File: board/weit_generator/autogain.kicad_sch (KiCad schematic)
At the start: 10 parts, among them U1 MCP6004, U3 LM4041LP-ADJ

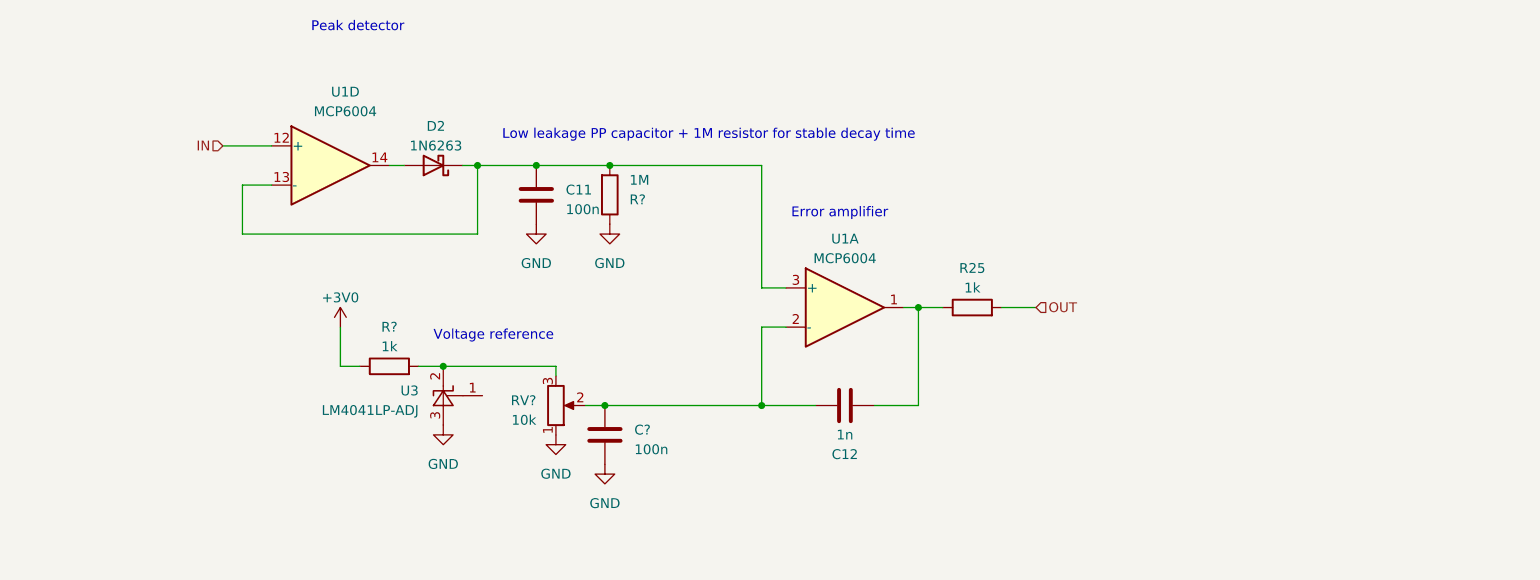
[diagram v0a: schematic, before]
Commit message: hopefully repaired instability
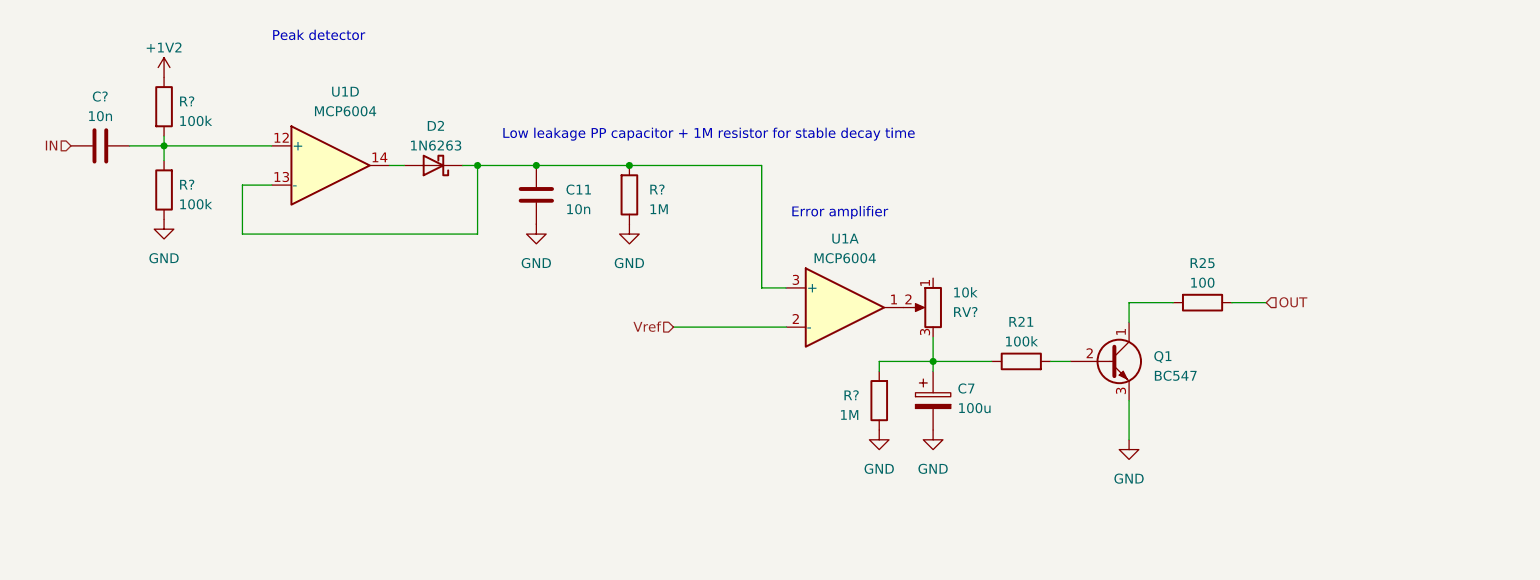
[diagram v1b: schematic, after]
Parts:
- removed C12: 1n, Capacitor_SMD:C_0805_2012Metric_Pad1.18x1.45mm_HandSolder, symbol Device:C
- removed C?: 100n, Capacitor_SMD:C_0805_2012Metric_Pad1.18x1.45mm_HandSolder, symbol Device:C
- removed R?: 1k, Resistor_SMD:R_0805_2012Metric_Pad1.20x1.40mm_HandSolder, symbol Device:R
- removed RV?: 10k, Potentiometer_THT:Potentiometer_Bourns_3266Y_Vertical, symbol Device:R_Potentiometer
- removed U3: LM4041LP-ADJ, Package_TO_SOT_THT:TO-92_Inline, symbol Reference_Voltage:LM4041LP-ADJ
- added C7: 100u, symbol Device:C_Polarized
- added C?: 10n, Capacitor_THT:C_Rect_L9.0mm_W4.0mm_P7.50mm_MKT, symbol Device:C
- added Q1: BC547, Package_TO_SOT_THT:TO-92_Inline, symbol Transistor_BJT:BC547
- added R21: 100k, Resistor_THT:R_Axial_DIN0207_L6.3mm_D2.5mm_P2.54mm_Vertical, symbol Device:R
- added R?: 1M, Resistor_THT:R_Axial_DIN0207_L6.3mm_D2.5mm_P2.54mm_Vertical, symbol Device:R
- added R? (x2): 100k, Resistor_SMD:R_0805_2012Metric_Pad1.20x1.40mm_HandSolder, symbol Device:R
- added RV?: 10k, Potentiometer_THT:Potentiometer_Bourns_3266Y_Vertical, symbol Device:R_Potentiometer
- C11: value 100n -> 10n
- R25: value 1k -> 100
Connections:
- net GND: now also C7.2, Q1.3 (E), R?.1, R?.1
- net IN: now also C?.2; no longer U1.12 (+)
- net OUT: now also R25.1; no longer R25.2
- net at U1.1: now also RV?.2; no longer R25.1
- net Vref: now reaches U1.2 (-)
- new net: C7.1, R21.1, R?.2, RV?.3
- new net: C?.1, R?.2, R?.2, U1.12 (+)
- new net: Q1.1 (C), R25.2
- new net: Q1.2 (B), R21.2
- new net +1V2: R?.1
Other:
- note removed: "Voltage reference"
- moved on the sheet: R25, R?

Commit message: New layout
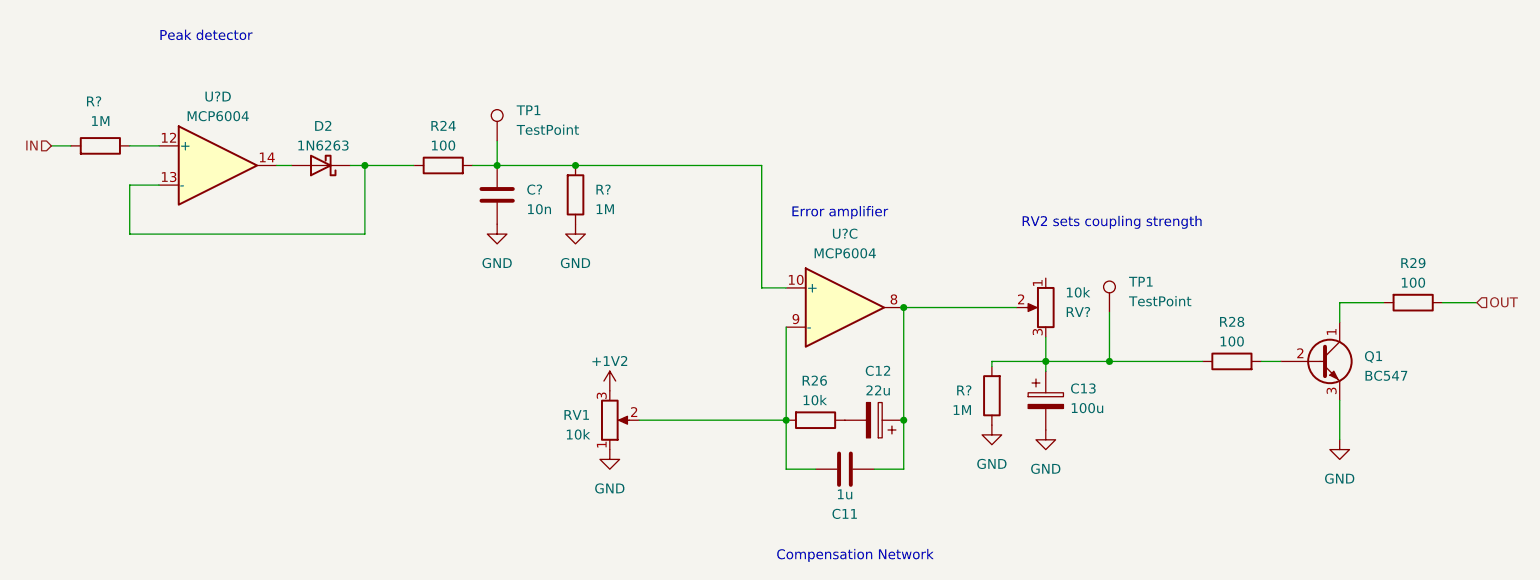
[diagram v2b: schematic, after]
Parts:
- removed C?: 10n, Capacitor_THT:C_Rect_L9.0mm_W4.0mm_P7.50mm_MKT, symbol Device:C
- removed R? (x2): 100k, Resistor_SMD:R_0805_2012Metric_Pad1.20x1.40mm_HandSolder, symbol Device:R
- removed U1: MCP6004, Package_DIP:DIP-14_W7.62mm_Socket_LongPads, symbol Amplifier_Operational:MCP6004
- added C11: 1u, Capacitor_THT:C_Rect_L7.2mm_W4.5mm_P5.00mm_FKS2_FKP2_MKS2_MKP2, symbol Device:C
- added C12: 22u, Capacitor_THT:CP_Radial_D6.3mm_P2.50mm, symbol Device:C_Polarized
- added R24: 100, Resistor_THT:R_Axial_DIN0207_L6.3mm_D2.5mm_P2.54mm_Vertical, symbol Device:R
- added R26: 10k, Resistor_THT:R_Axial_DIN0207_L6.3mm_D2.5mm_P2.54mm_Vertical, symbol Device:R
- added R?: 1M, Resistor_THT:R_Axial_DIN0207_L6.3mm_D2.5mm_P2.54mm_Vertical, symbol Device:R
- added RV1: 10k, Potentiometer_THT:Potentiometer_Bourns_3266Y_Vertical, symbol Device:R_Potentiometer
- added TP1 (x2): TestPoint, TestPoint:TestPoint_Pad_D3.0mm, symbol Connector:TestPoint
- added U? (x2): MCP6004, Package_DIP:DIP-14_W7.62mm_Socket, symbol Amplifier_Operational:MCP6004
- C13: renamed from C7; footprint (none) -> Capacitor_THT:CP_Radial_D6.3mm_P2.50mm
- C?: renamed from C11; footprint Capacitor_THT:C_Rect_L13.0mm_W6.0mm_P10.00mm_FKS3_FKP3_MKS4 -> Capacitor_THT:C_Rect_L13.0mm_W4.0mm_P10.00mm_FKS3_FKP3_MKS4; Dielectric (none) -> Polistyrene
- R28: renamed from R21; value 100k -> 100
- renumbered R25 to R29
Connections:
- net +1V2: now also RV1.3
- net GND: now also RV1.1
- net IN: now also R?.2
- net at C?.2, R?.2: now also R24.2, TP1.1, U?.10 (+); no longer D2.1 (K)
- net at C13.1, R28.1, R?.2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: now also TP1.1
- net at D2.2 (A): now also U?.14
- net at RV?.2: now also C11.2, C12.1, U?.8
- new net: D2.1 (K), R24.1, U?.13 (-)
- new net: C12.2, R26.1
- new net: C11.1, R26.2, RV1.2, U?.9 (-)
- new net: R?.1, U?.12 (+)
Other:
- note added: "Compensation Network"
- note added: "RV2 sets coupling strength"
- note removed: "Low leakage PP capacitor + 1M resistor for stable decay time"
- moved on the sheet: C13, C?, D2, Q1, R28, R29, R?, RV?
